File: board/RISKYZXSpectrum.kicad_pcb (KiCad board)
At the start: 4 copper layers, 77.1 x 87.5 mm, 31 parts, among them J1 Conn_01x02, J2 Conn_01x02, J3 Conn_02x28_Odd_Even, J4 Conn_02x28_Odd_Even, J7 USB_1, J8 Conn_01x02, SW1 SW_SPST, SW2 SW_SPST, U1 CH32V307VCT6, U2 LM1117MP-3.3

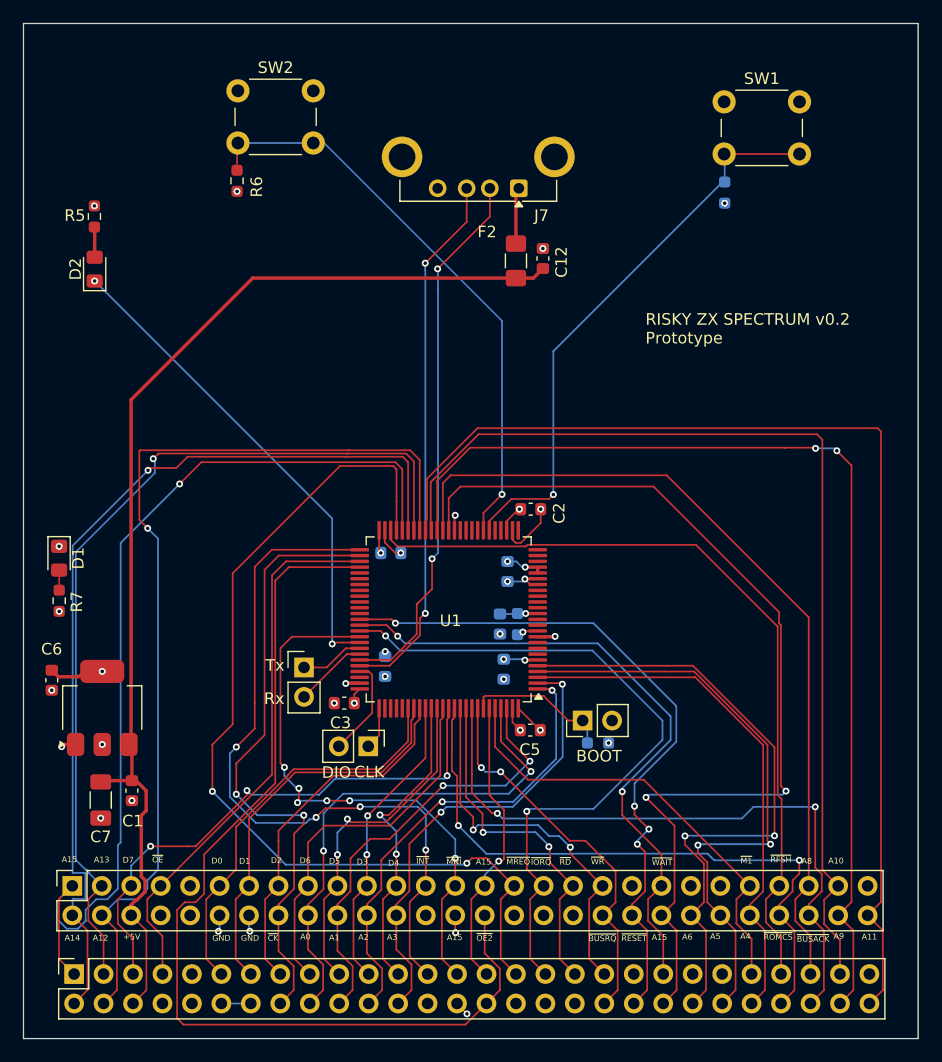
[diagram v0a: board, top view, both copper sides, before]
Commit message: PCB udpate
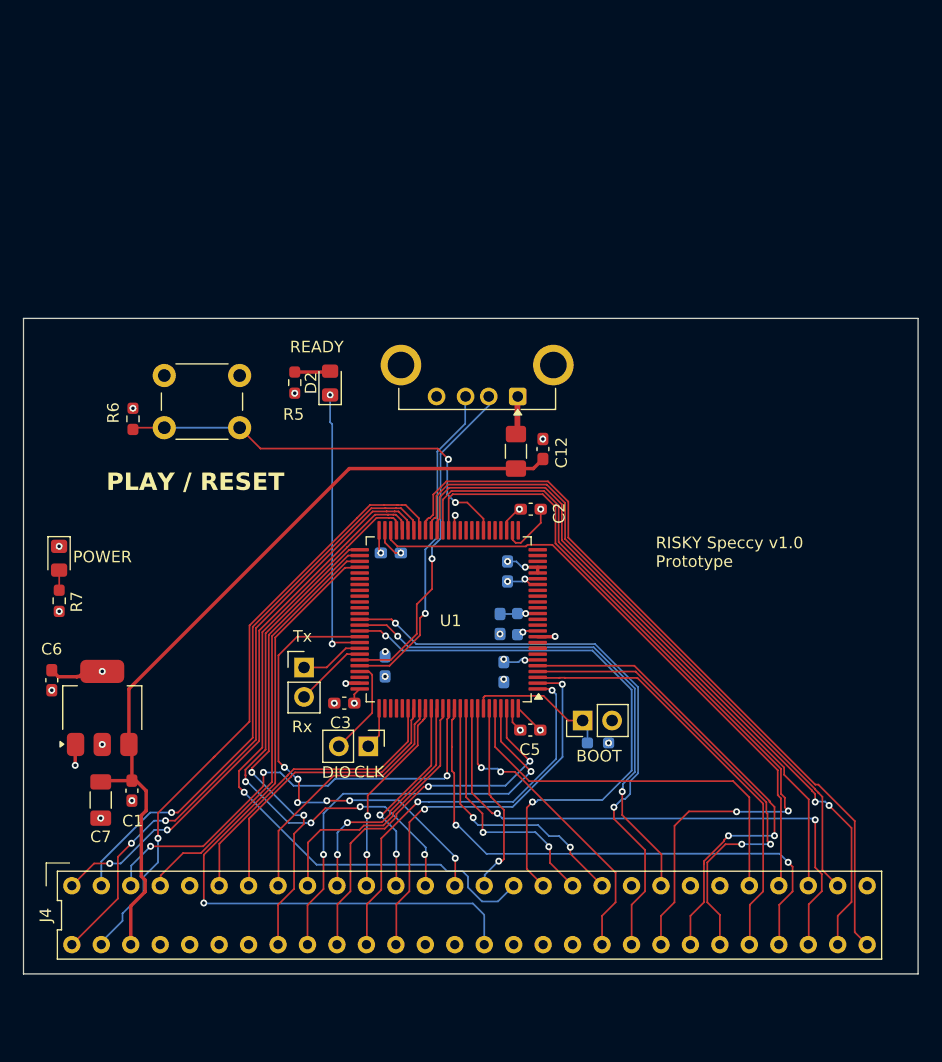
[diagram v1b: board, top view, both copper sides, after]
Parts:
- removed J3: Conn_02x28_Odd_Even, Connector_PinSocket_2.54mm:PinSocket_2x28_P2.54mm_Vertical
- removed R2: R, Resistor_SMD:R_0603_1608Metric_Pad0.98x0.95mm_HandSolder
- removed the SW1 at (155.5, 63.4)
- J4: footprint Connector_PinSocket_2.54mm:PinSocket_2x28_P2.54mm_Vertical -> edgeconnector:EdgeConnector_254x508x2x28_OddEven
- moved J4 34.3 mm to (133.5, 133.6), turned to 0 degrees
- moved SW1 25.4 mm to (107.2, 87.0)
- moved D2 22.6 mm to (121.5, 87.7)
- moved R5 22.4 mm to (118.5, 87.6), turned to -90 degrees
- moved R6 22.4 mm to (104.5, 90.8), turned to 90 degrees
- moved J7 18.0 mm to (137.7, 88.8)
- moved C12 16.4 mm to (139.8, 93.4)
- moved F2 16.4 mm to (137.5, 93.6)
- moved C11 0.25 mm to (136.5, 112.6)
- renumbered SW2 to SW1
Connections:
- R6 pad 1: /BTN2 -> /BTN1
- SW1 pad 2: /BTN2 -> /BTN1
- U1 pad 31: /BTN1 -> unconnected-(U1-PA6/ADC6-Pad31)
- U1 pad 32: /BTN2 -> /BTN1
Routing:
- net /BTN2: track 50.2 -> 0.00 mm, vias 1 -> 0
- net /A15: track 82.1 -> 48.3 mm, vias 1 -> 2
- net /A11: track 96.4 -> 65.3 mm
- net /A12: track 82.9 -> 53.0 mm
- net /A13: track 78.2 -> 48.4 mm
- net /A10: track 87.6 -> 58.1 mm
- net +5V: track 97.6 -> 69.2 mm
- net /A14: track 80.9 -> 53.2 mm, vias 1 -> 2
- net /A9: track 89.7 -> 63.7 mm
- net /~{OE2}: track 85.8 -> 62.3 mm, vias 0 -> 1
- net /~{MREQ}: track 81.4 -> 59.5 mm, vias 2 -> 1
- net /LEDFLASH: track 42.2 -> 24.0 mm
- net /USB1_DM: track 46.9 -> 28.9 mm, vias 2 -> 1
- net /USB1_DP: track 46.5 -> 28.5 mm, vias 2 -> 1
- net /A8: track 72.7 -> 55.2 mm
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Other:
- board size 77.1 x 87.5 mm -> 77.1 x 56.5 mm
- board text added: "PLAY / RESET"
- board text added: "POWER"
- board text added: "READY"
- board text added: "RISKY Speccy v1.0 Prototype"
- board text removed: "+5V"
- board text removed: "A0"
- board text removed: "A1"
- board text removed: "A10"
- board text removed: "A11"
- board text removed: "A12"
- board text removed: "A13"
- board text removed: "A14"
- board text removed: "A15"
- board text removed: "A2"
- board text removed: "A3"
- board text removed: "A4"
- board text removed: "A5"
- board text removed: "A6"
- board text removed: "A8"
- board text removed: "A9"
- board text removed: "D0"
- board text removed: "D1"
- board text removed: "D2"
- board text removed: "D3"
- board text removed: "D4"
- board text removed: "D5"
- board text removed: "D6"
- board text removed: "D7"
- board text removed: "GND"
- board text removed: "RISKY ZX SPECTRUM v0.2 Prototype"
- board text removed: "~{BUSACK}"
- board text removed: "~{BUSRQ}"
- board text removed: "~{CK}"
- board text removed: "~{INT}"
- board text removed: "~{IORQ}"
- board text removed: "~{M1}"
- board text removed: "~{MNI}"
- board text removed: "~{MREQ}"
- board text removed: "~{OE2}"
- board text removed: "~{OE}"
- board text removed: "~{RD}"
- board text removed: "~{RESET}"
- board text removed: "~{RFSH}"
- board text removed: "~{ROMCS}"
- board text removed: "~{WAIT}"
- board text removed: "~{WR}"
